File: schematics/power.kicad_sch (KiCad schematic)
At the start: 42 parts, among them J1 9VRMS 60HZ AC, SW1 SW_SPDT, SW2 SW_Push, SW3 SW_Push, SW4 SW_Push, U1 74HC14, U2 LM2576T-ADJ, U3 LM317T, U5 74HC08

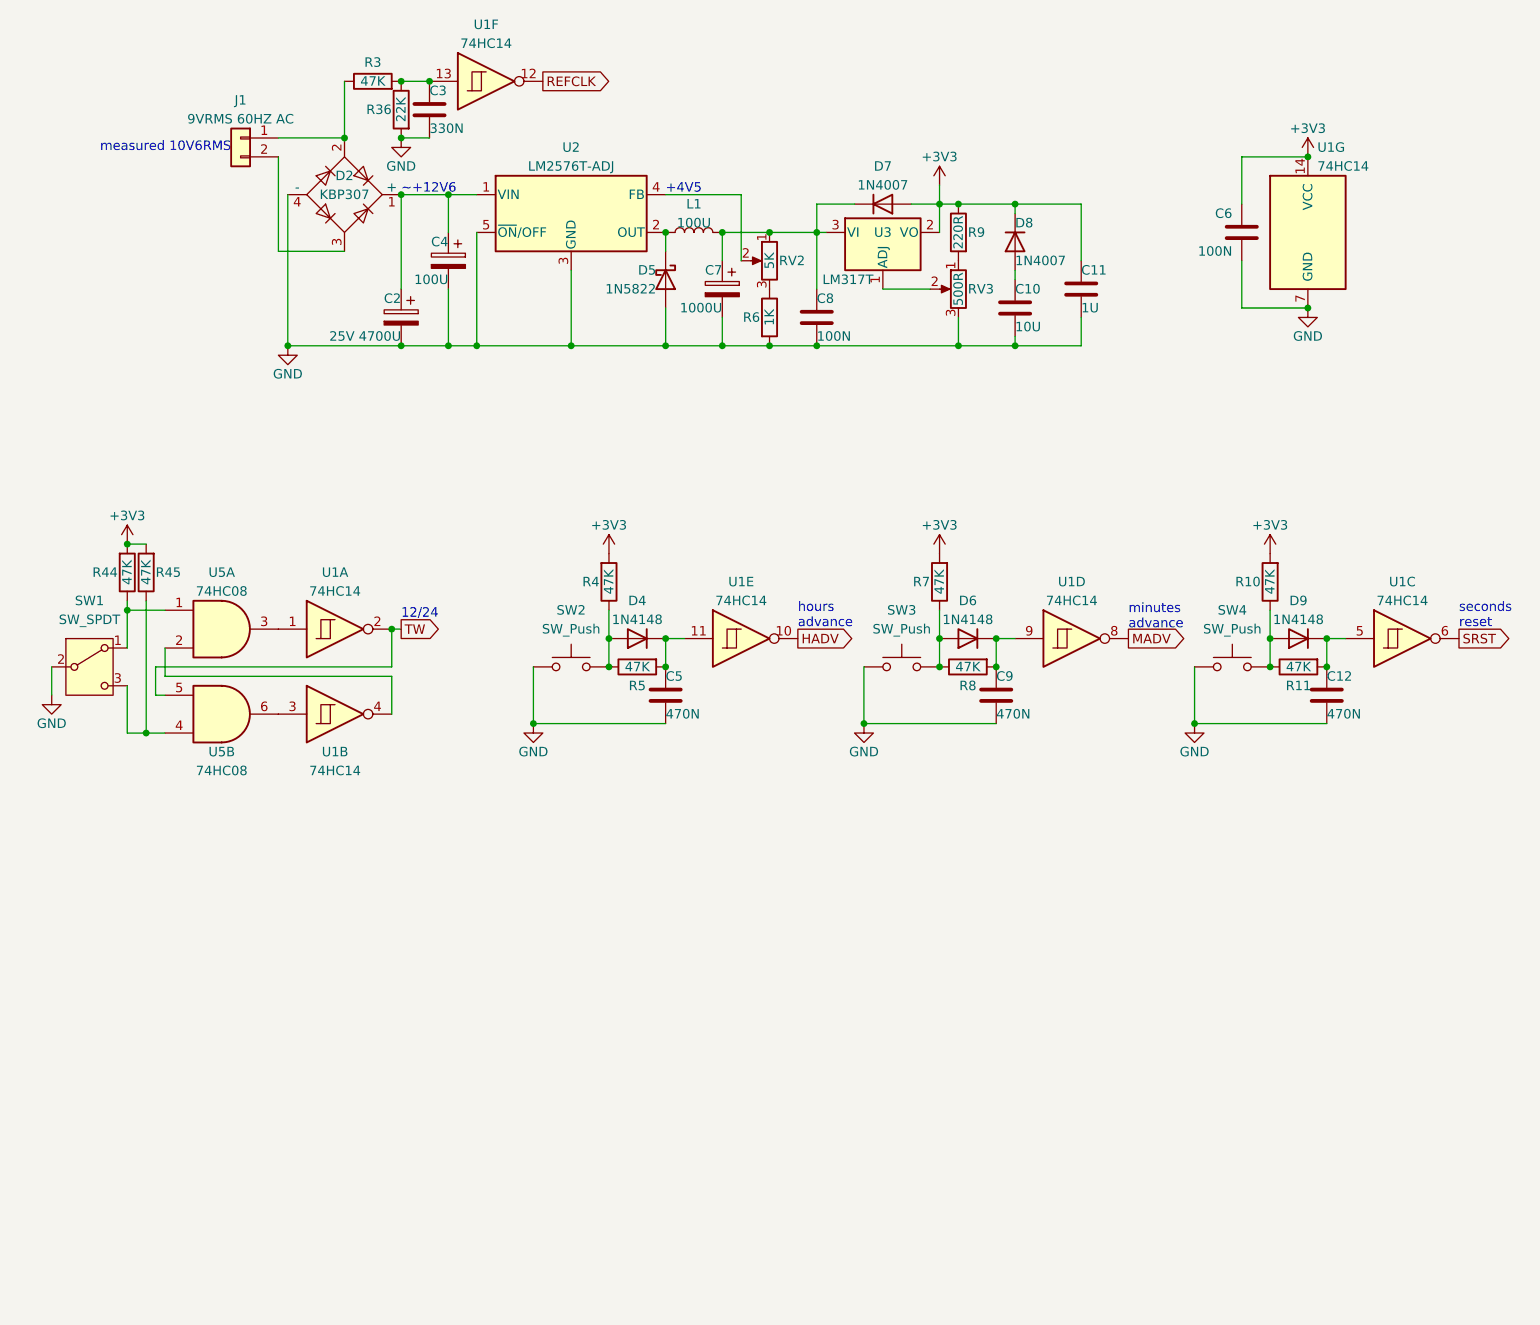
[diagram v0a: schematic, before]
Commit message: started a second version
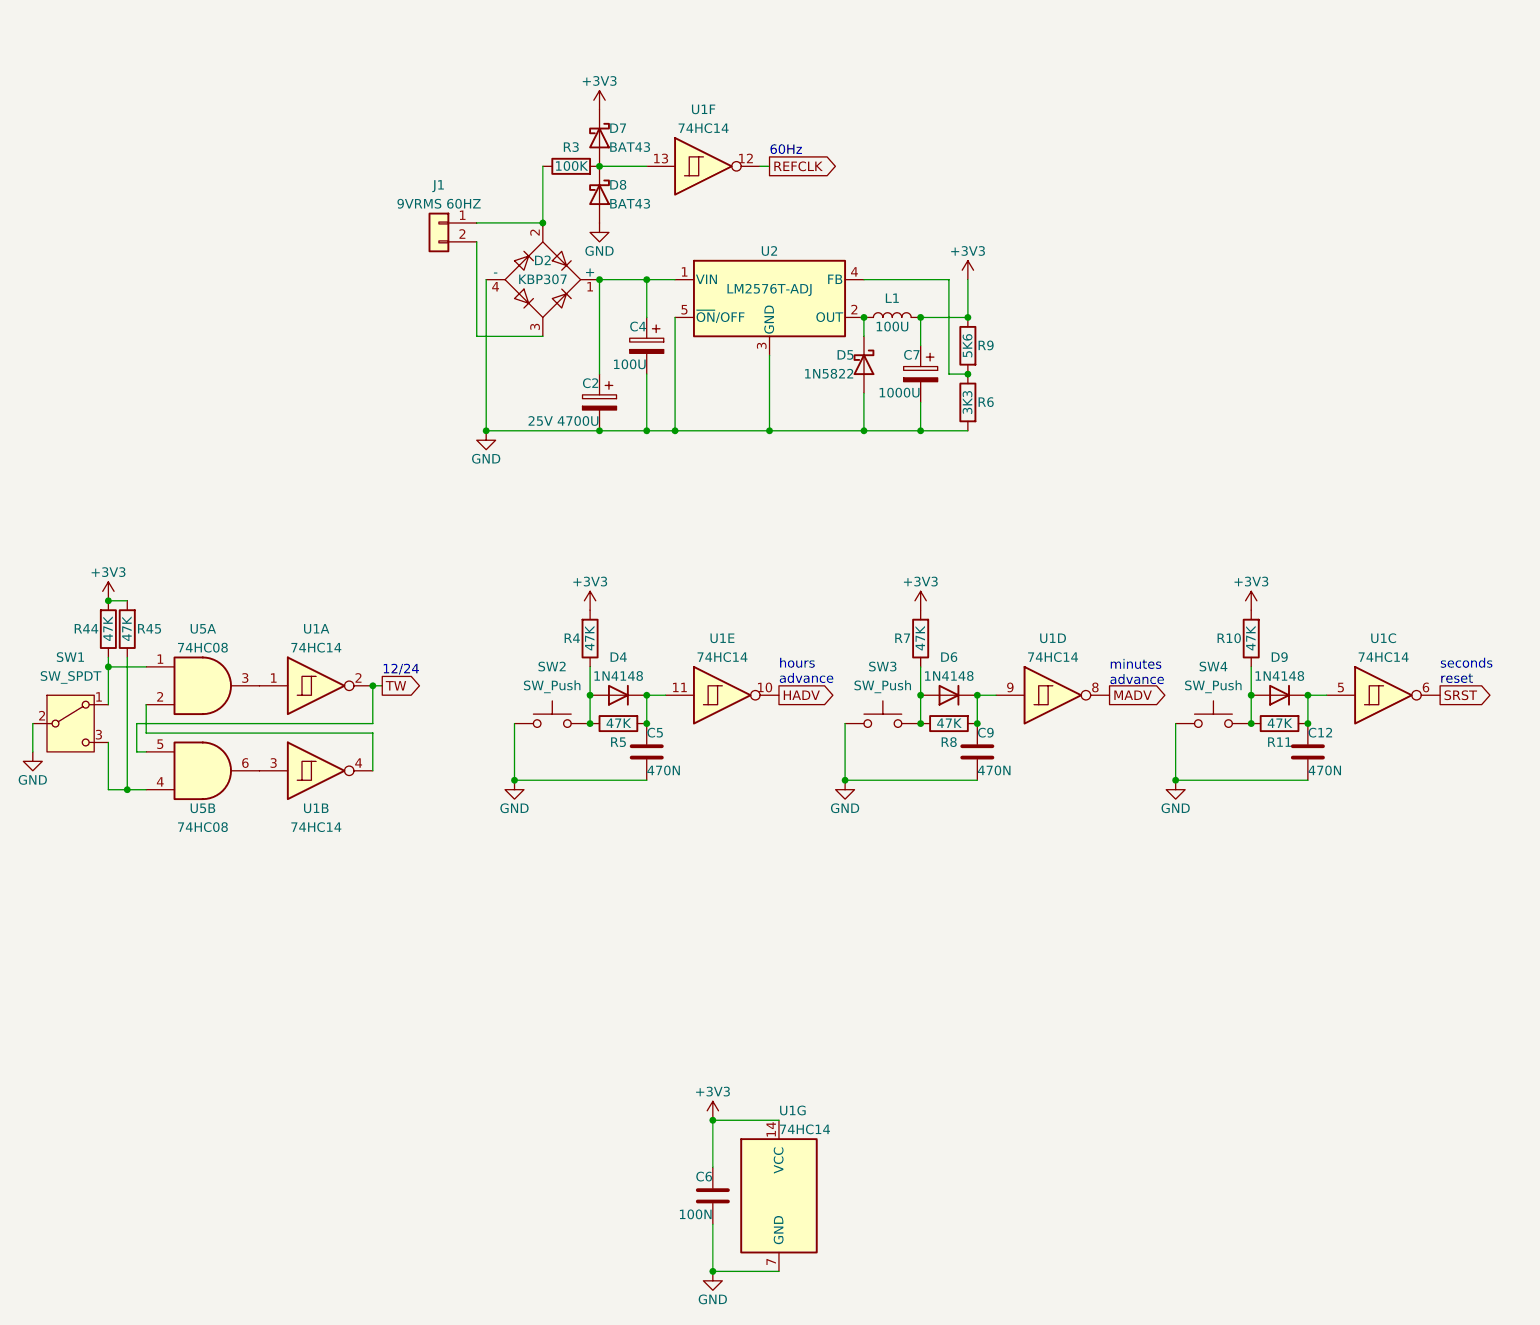
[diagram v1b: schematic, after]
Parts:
- removed C10: 10U, Package_SO:SOIC-8_3.9x4.9mm_P1.27mm, symbol Device:C
- removed C11: 1U, Package_SO:SOIC-8_3.9x4.9mm_P1.27mm, symbol Device:C
- removed C3: 330N, Package_SO:SOIC-8_3.9x4.9mm_P1.27mm, symbol Device:C
- removed C8: 100N, Package_SO:SOIC-8_3.9x4.9mm_P1.27mm, symbol Device:C
- removed D7, D8: 1N4007, Diode_THT:D_DO-35_SOD27_P7.62mm_Horizontal, symbol Diode:1N4148
- removed R36: 22K, symbol Device:R
- removed RV2: 5K, Package_SO:TSSOP-20_4.4x6.5mm_P0.65mm, symbol Device:R_Potentiometer
- removed RV3: 500R, Package_SO:TSSOP-20_4.4x6.5mm_P0.65mm, symbol Device:R_Potentiometer
- removed U3: LM317T, Package_TO_SOT_THT:TO-220-3_Vertical, symbol Regulator_Linear:LM317_TO-220
- added D7, D8: BAT43, Package_SON:WSON-8-1EP_6x5mm_P1.27mm_EP3.4x4mm, symbol Device:D_Schottky
- J1: value 9VRMS 60HZ AC -> 9VRMS 60HZ
- R3: value 47K -> 100K
- R6: value 1K -> 3K3
- R9: value 220R -> 5K6
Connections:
- net +3V3: now also C7.1, L1.2, D7.1 (K)
- net GND: now also D8.2 (A)
- net at R9.2: now also R6.1, U2.4 (FB)
- net at R3.2, U1.13: now also D7.2 (A), D8.1 (K)
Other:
- note added: "60Hz"
- note removed: "+4V5"
- note removed: "measured 10V6RMS"
- note removed: "~+12V6"
- moved on the sheet: C12, C2, C4, C5, C6, C7, C9, D2, D4, D5, D6, D9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
